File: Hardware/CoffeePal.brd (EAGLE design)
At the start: 28.1 x 40.6 mm, 27 parts, among them U1 ATTINY85SOIC-8, U2 BH1745NUC-E2WSON008X2120, U3 TP143305-1PIETZO, U4 CMPT3904ETRPBFREESOT23

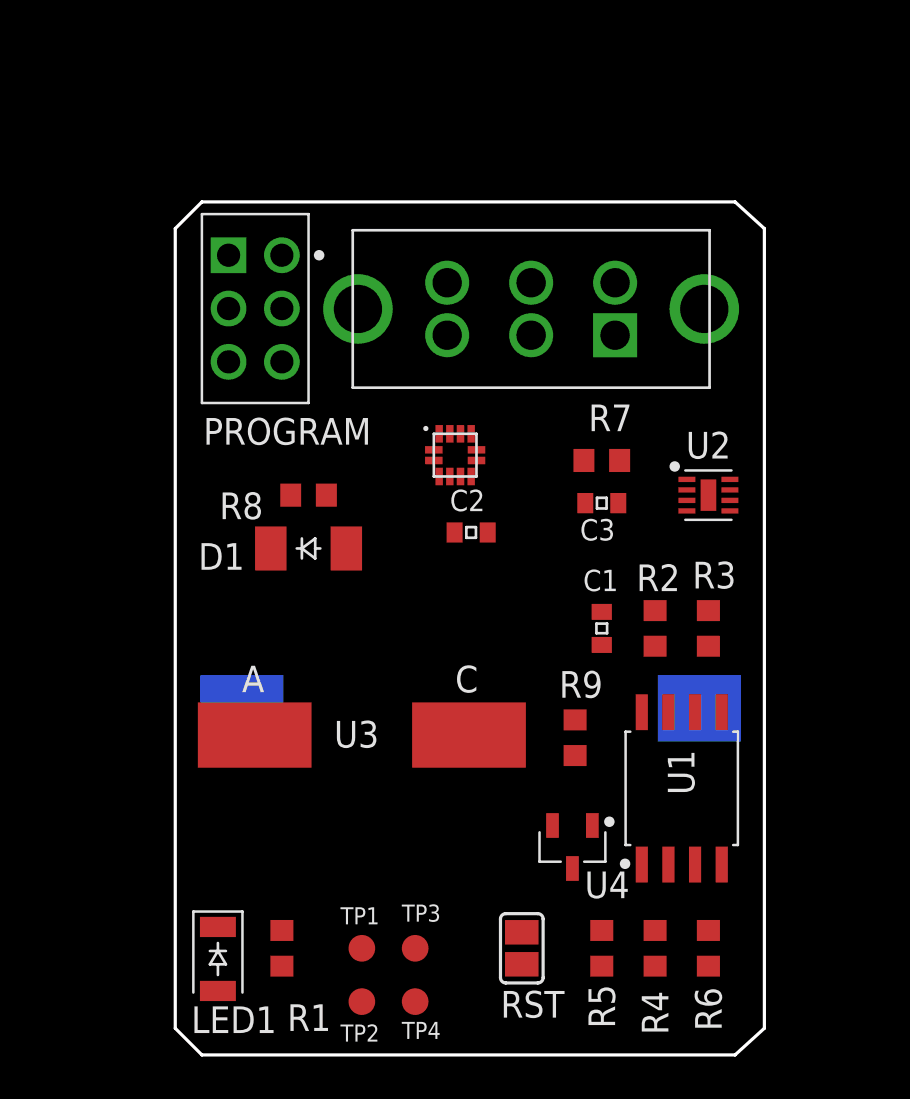
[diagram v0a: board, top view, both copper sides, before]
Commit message: Drew traces and created boom
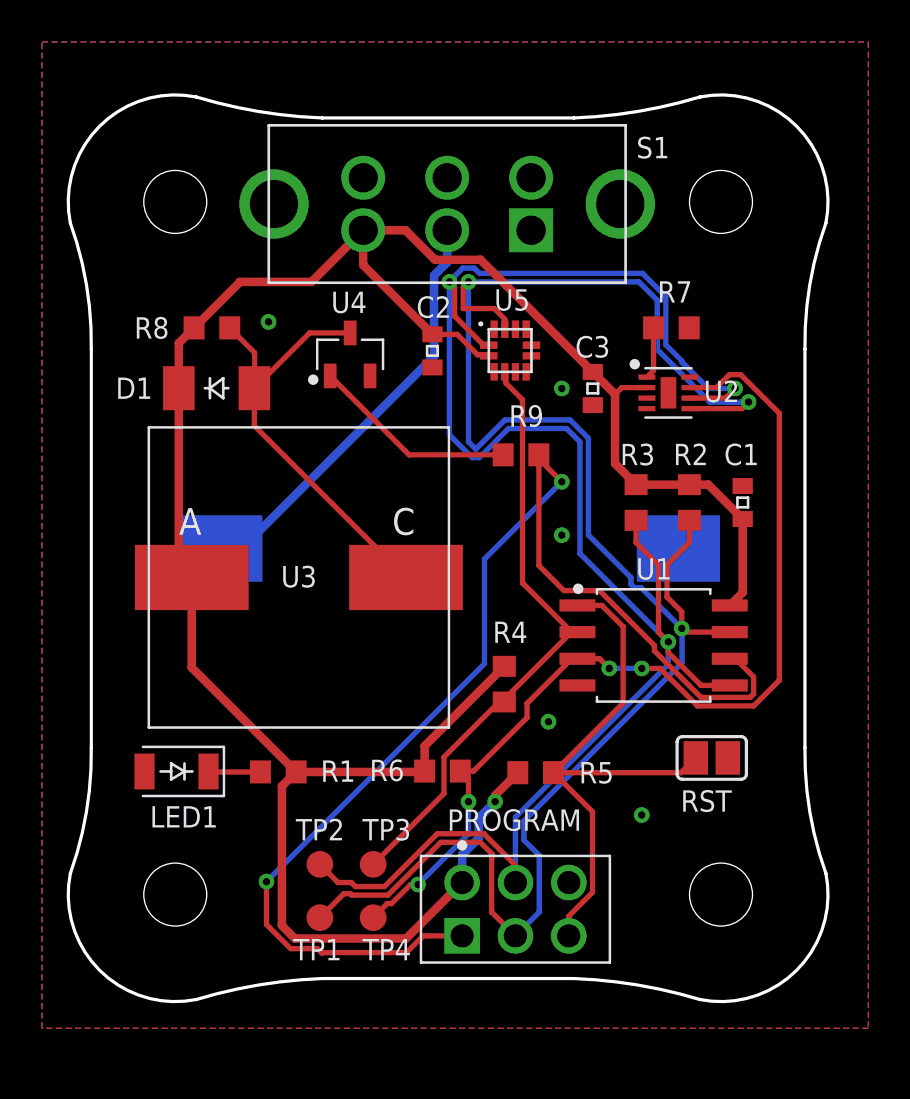
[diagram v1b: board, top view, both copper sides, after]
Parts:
- removed U$1: MC3413, lib:VLGA-12
- added U$3: UTBULT_DESIGN1, lib:UD_1
- added U5: MC3413, lib:VLGA-12
- D1: value DIODE1 -> 1N4448W-7-F
- moved PROGRAM 31.1 mm to (13.7, -32.4), turned to 0 degrees
- moved U4 25.7 mm to (8.33, -7.27), turned to 90 degrees
- moved R6 15.2 mm to (12.7, -27.1), turned to 0 degrees
- moved R4 14.5 mm to (15.7, -23.0), turned to 270 degrees
- moved R9 13.7 mm to (16.5, -12.1), turned to 180 degrees
- moved RST 12.8 mm to (25.6, -26.5), turned to 180 degrees
- moved R8 9.20 mm to (1.75, -6.00)
- moved LED1 9.15 mm to (0.06, -27.1), turned to 180 degrees
- moved C1 9.01 mm to (27.0, -14.3)
- moved R5 8.94 mm to (17.2, -27.2), turned to 0 degrees
- moved C2 8.85 mm to (12.3, -7.10), turned to 90 degrees
- moved D1 8.80 mm to (1.97, -8.88)
- moved R1 8.40 mm to (4.91, -27.2), turned to 0 degrees
- moved U3 8.09 mm to (5.89, -17.9)
- moved U$2 7.68 mm to (13.0, -16.5)
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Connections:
- removed net SCL/SCK: PROGRAM.2, R2.2, TP1.TP, U$1.P$12, U1.7, U2.5
- removed net SDA/MOSI: PROGRAM.5, R3.2, TP2.TP, U$1.P$2, U1.5, U2.6
- new net I2C_N: PROGRAM.5, R3.2, TP2.TP, U1.5, U2.6, U5.P$2
- new net I2C_P: PROGRAM.2, R2.2, TP1.TP, U1.7, U2.5, U5.P$12
- net +3V3: now also U5.P$3; no longer U$1.P$3
- net GND: now also U5.P$6, U5.P$9; no longer U$1.P$6, U$1.P$9
- net INT0: now also U5.P$5; no longer U$1.P$5
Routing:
- net +3V3: track 0.00 -> 111.9 mm, vias 0 -> 1
- net I2C_P: track 0.00 -> 90.7 mm, vias 0 -> 3
- net I2C_N: track 0.00 -> 87.2 mm, vias 0 -> 3
- net PWM/MISO: track 0.00 -> 59.5 mm, vias 0 -> 2
- net INT1: track 0.00 -> 46.6 mm, vias 0 -> 4
- net INT0: track 0.00 -> 29.4 mm
- net RST: track 0.00 -> 27.0 mm
- net N$7: track 0.00 -> 21.0 mm
- net N$1: track 0.00 -> 20.2 mm
- net N$6: track 0.00 -> 9.80 mm
- net N$2: track 0.00 -> 2.48 mm
- net N$4: track 0.00 -> 2.48 mm
- added copper zone on layer 1, net GND
- added copper zone on layer 16, net GND
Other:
- board size 28.1 x 40.6 mm -> 36.2 x 43.2 mm
- board text added: "Coffee Pal"
